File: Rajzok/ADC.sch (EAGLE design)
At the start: 17 parts, among them Q1 TP0602N2, Q2 TP0602N2, Q3 SUP75N06-08, Q4 SUP75N06-08

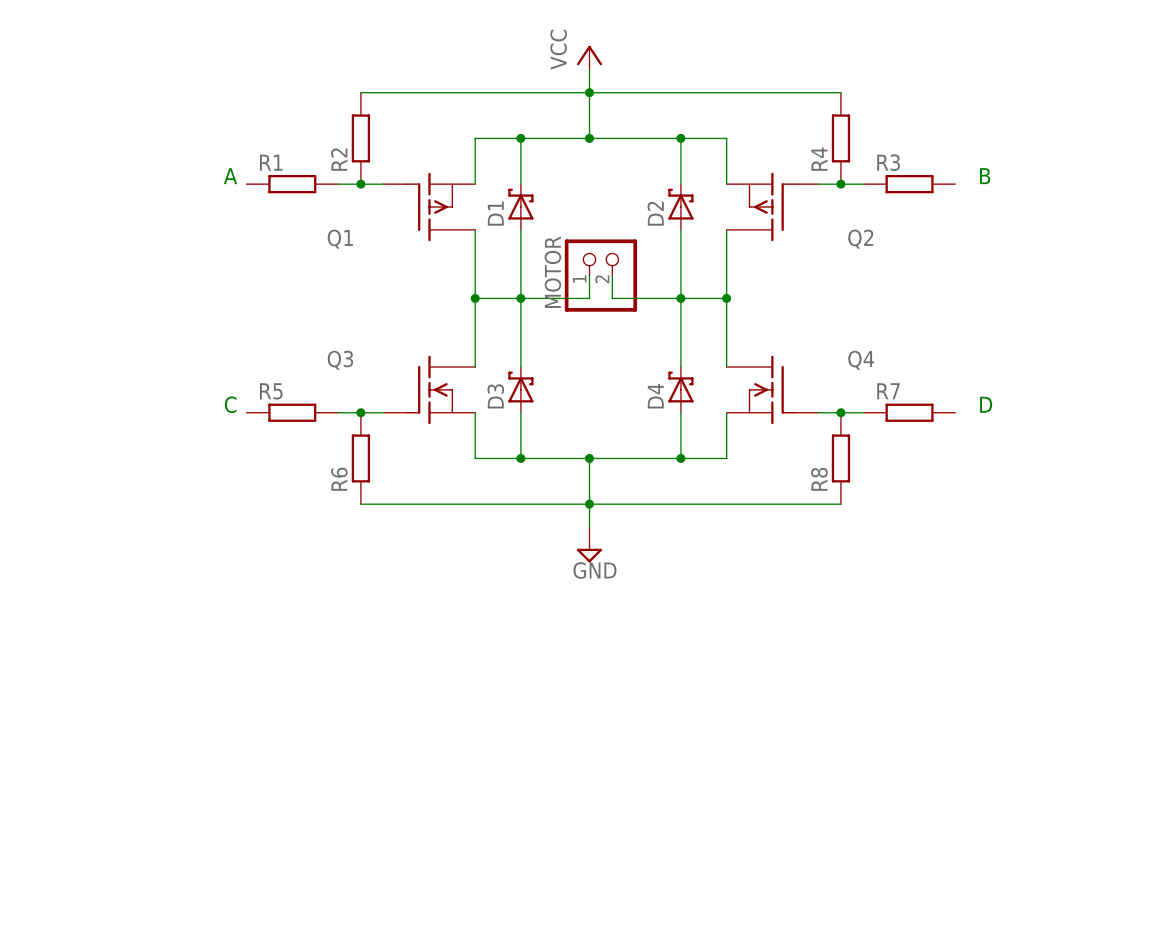
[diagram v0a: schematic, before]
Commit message: Rajzok 2017
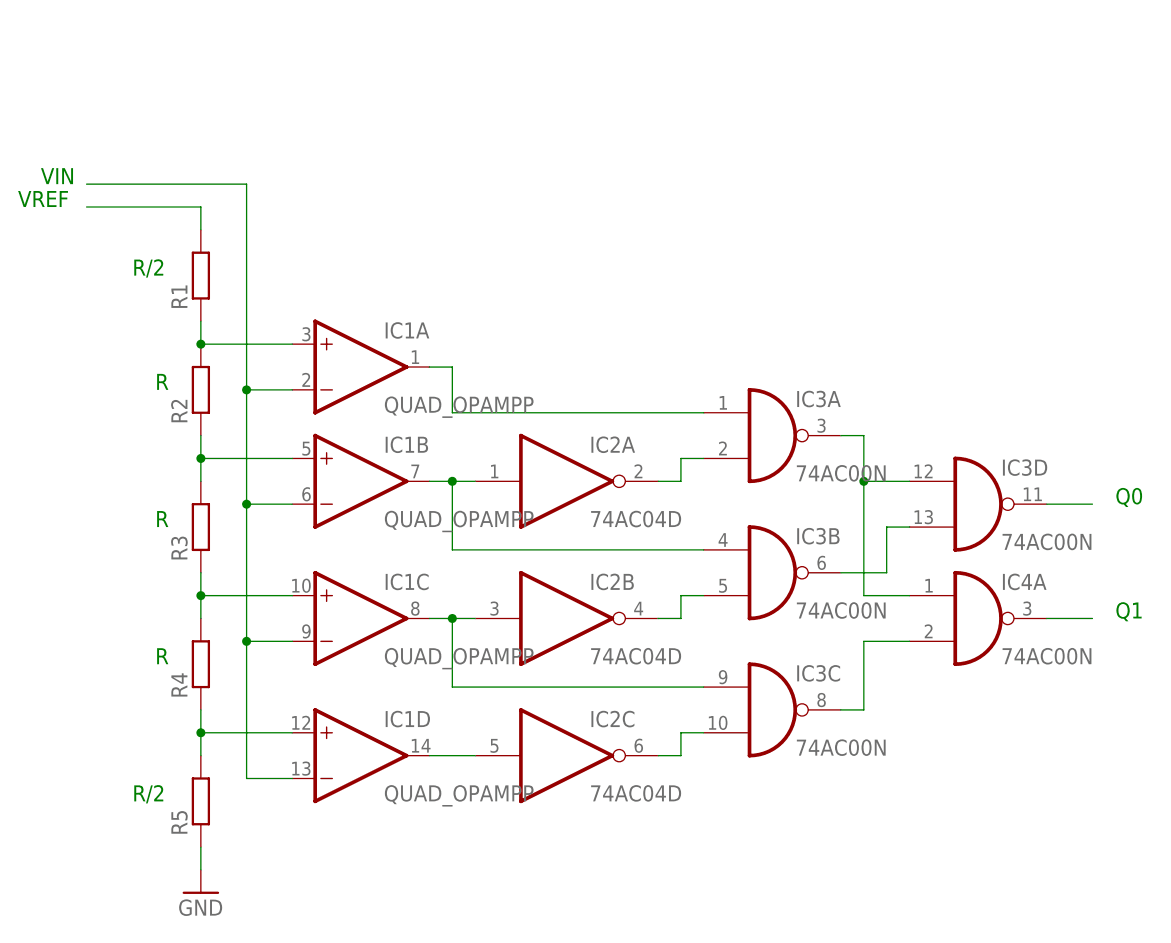
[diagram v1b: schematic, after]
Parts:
- removed D1, D2, D3, D4: 1N6267A, diode:1N6267A
- removed MOTOR: (no value), pinhead:PINHD-1X2
- removed Q1, Q2: TP0602N2, transistor-fet:TP0602N2
- removed Q3, Q4: SUP75N06-08, transistor-fet:SUP75N06-08
- removed R6, R7, R8: (no value), rcl:R-EU_0204/7
- added IC1: QUAD_OPAMPP, adafruit:QUAD_OPAMPP
- added IC2: 74AC04D, 74xx-eu:74AC04D
- added IC3, IC4: 74AC00N, 74xx-eu:74AC00N
- R1, R2, R3, R4, R5: device rcl:R-EU_0204/7 -> rcl:R-EU_0207/15
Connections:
- removed net VCC: D1.C, D2.C, Q1.S, Q2.S, R2.2, R4.2
- new net N$10: IC1A.OUT, IC3A.I0
- new net N$11: IC2B.O, IC3B.I1
- new net N$12: IC2C.O, IC3C.I1
- new net N$13: IC3A.O, IC3D.I0, IC4A.I0
- new net N$14: IC3C.O, IC4A.I1
- new net N$15: IC3B.O, IC3D.I1
- new net N$16: R1.2
- new net N$17: IC3D.O
- new net N$18: IC4A.O
- new net N$6: IC1D.OUT, IC2C.I
- new net N$7: IC2A.O, IC3A.I1
- new net N$8: IC1C.OUT, IC2B.I, IC3C.I0
- net GND: now also R5.1; no longer D3.A, D4.A, Q3.S, Q4.S, R6.1, R8.1
- net N$1: now also IC1A.-IN, IC1B.-IN, IC1C.-IN, IC1D.-IN; no longer Q1.G, R1.2, R2.1
- net N$2: now also IC1A.+IN, R1.1, R2.2; no longer D2.A, D4.C, MOTOR.2, Q2.D, Q4.D
- net N$3: now also IC1B.+IN, R2.1, R3.2; no longer Q2.G, R3.1, R4.1
- net N$4: now also IC1C.+IN, R3.1, R4.2; no longer Q3.G, R5.2, R6.2
- net N$5: now also IC1D.+IN, R4.1, R5.2; no longer Q4.G, R7.1, R8.2
- net N$9: now also IC1B.OUT, IC2A.I, IC3B.I0; no longer D1.A, D3.C, MOTOR.1, Q1.D, Q3.D
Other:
- note added: "Q0"
- note added: "Q1"
- note added: "R"
- note added: "R/2"
- note added: "VIN"
- note added: "VREF"
- note removed: "A"
- note removed: "B"
- note removed: "C"
- note removed: "D"
- moved on the sheet: R1, R2, R3, R4, R5
